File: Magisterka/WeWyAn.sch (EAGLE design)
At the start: 88 parts, among them IC1 LM324N, IC3 7805TV, IC4 LM324N, IC5 LM1117T-3.3-V, X10 22-23-2041, X11 22-23-2041, X18 22-23-2031, X19 22-23-2041, X20 22-23-2041, X21 22-23-2041, X28 22-23-2021, X29 22-23-2021, X30 22-23-2021, X31 22-23-2031, X4 22-23-2021

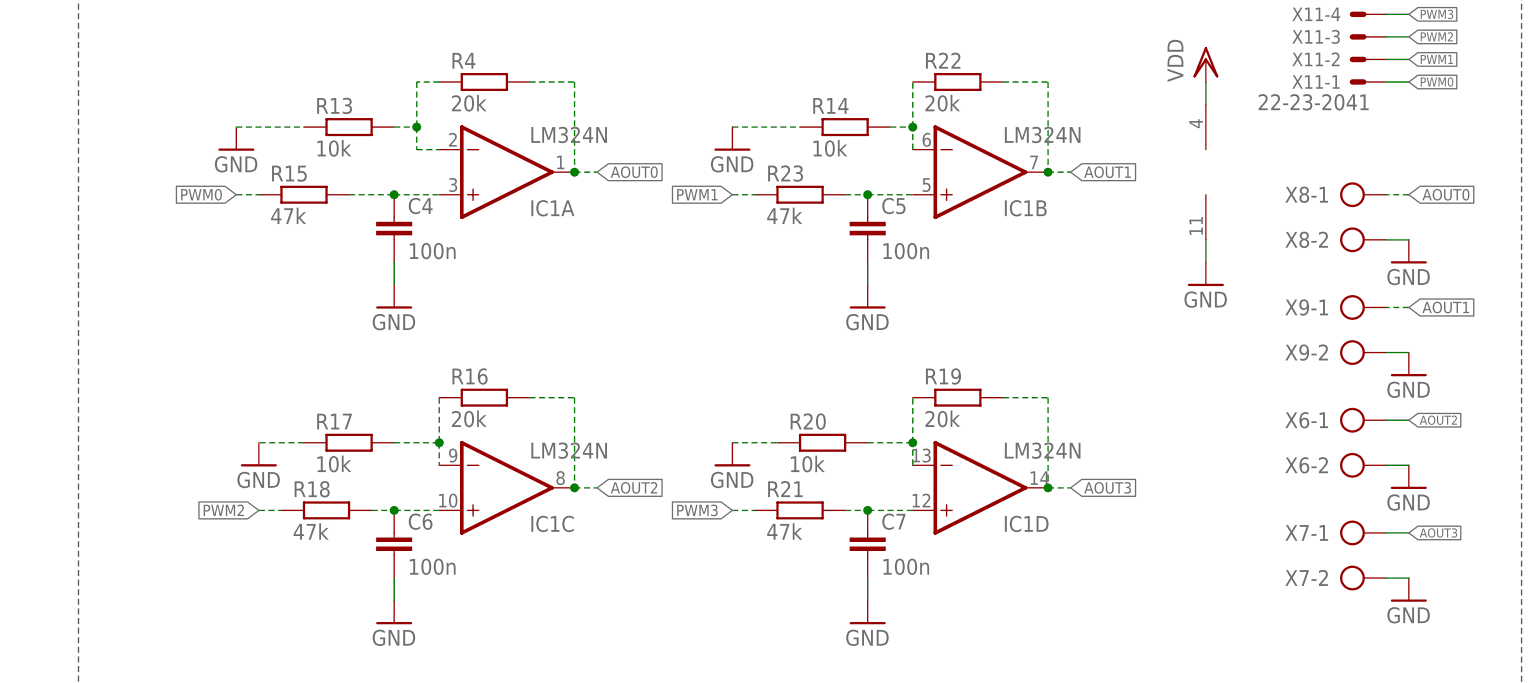
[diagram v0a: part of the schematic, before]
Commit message: size changes
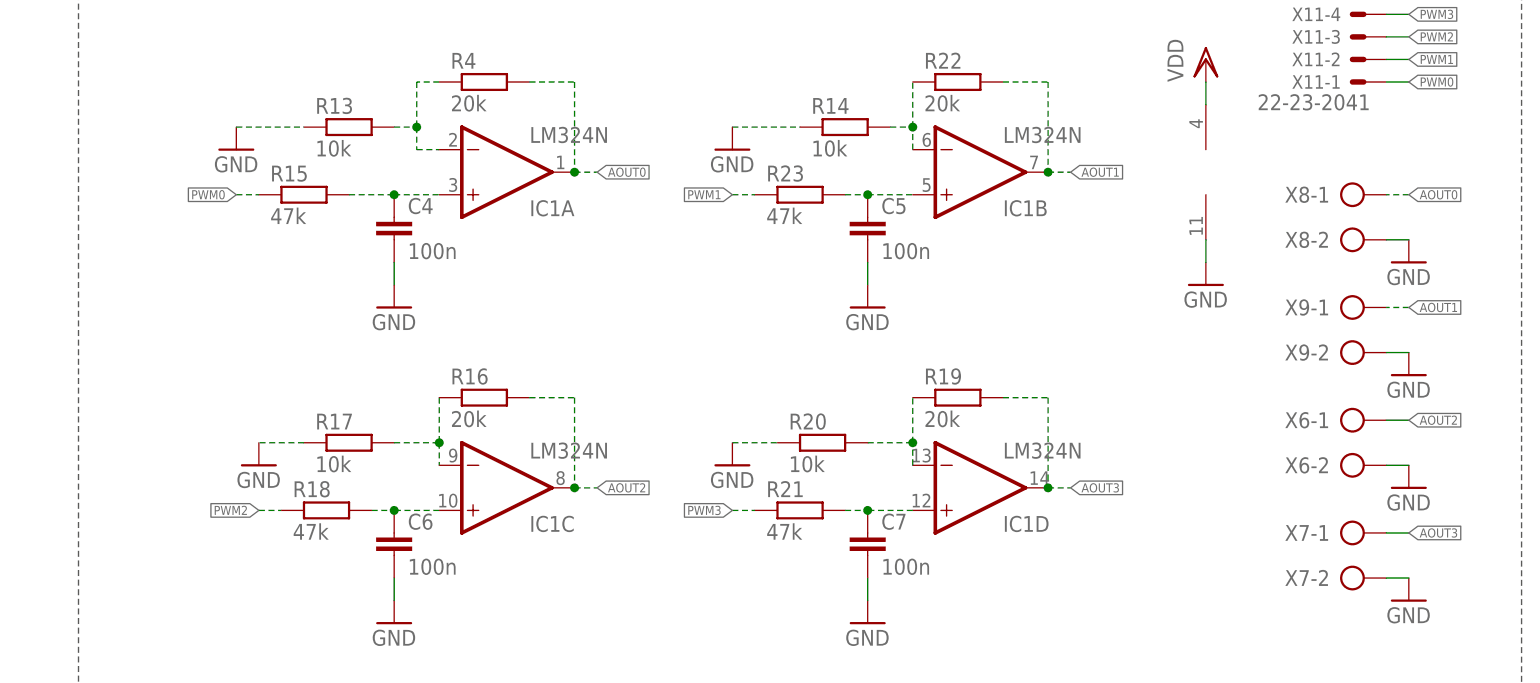
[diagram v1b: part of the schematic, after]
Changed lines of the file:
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@@
 <wire x1="261.62" y1="-30.48" x2="264.16" y2="-30.48" width="0.1524" layer="91" style="longdash"/>
 <junction x="261.62" y="-30.48"/>
-<label x="264.16" y="-30.48" size="1.27" layer="95" xref="yes"/>
+<label x="264.16" y="-30.48" size="1.016" layer="95" xref="yes"/>
 </segment>
 <segment>
 <pinref part="X8" gate="-1" pin="KL"/>
 <wire x1="355.6" y1="-33.02" x2="353.06" y2="-33.02" width="0.1524" layer="91" style="longdash"/>
-<label x="355.6" y="-33.02" size="1.27" layer="95" xref="yes"/>
+<label x="355.6" y="-33.02" size="1.016" layer="95" xref="yes"/>
 </segment>
 </net>
@@
 <pinref part="R15" gate="G$1" pin="1"/>
 <wire x1="223.52" y1="-33.02" x2="226.06" y2="-33.02" width="0.1524" layer="91" style="longdash"/>
-<label x="223.52" y="-33.02" size="1.27" layer="95" rot="R180" xref="yes"/>
+<label x="223.52" y="-33.02" size="1.016" layer="95" rot="R180" xref="yes"/>
 </segment>
 <segment>
@@
 <wire x1="261.62" y1="-66.04" x2="264.16" y2="-66.04" width="0.1524" layer="91" style="longdash"/>
 <junction x="261.62" y="-66.04"/>
-<label x="264.16" y="-66.04" size="1.27" layer="95" xref="yes"/>
+<label x="264.16" y="-66.04" size="1.016" layer="95" xref="yes"/>
 </segment>
 <segment>
@@
 <wire x1="314.96" y1="-66.04" x2="317.5" y2="-66.04" width="0.1524" layer="91" style="longdash"/>
 <junction x="314.96" y="-66.04"/>
-<label x="317.5" y="-66.04" size="1.27" layer="95" xref="yes"/>
+<label x="317.5" y="-66.04" size="1.016" layer="95" xref="yes"/>
 </segment>
 <segment>
@@
 <pinref part="R18" gate="G$1" pin="1"/>
 <wire x1="226.06" y1="-68.58" x2="228.6" y2="-68.58" width="0.1524" layer="91" style="longdash"/>
-<label x="226.06" y="-68.58" size="1.27" layer="95" rot="R180" xref="yes"/>
+<label x="226.06" y="-68.58" size="1.016" layer="95" rot="R180" xref="yes"/>
 </segment>
 <segment>
@@
 <pinref part="R21" gate="G$1" pin="1"/>
 <wire x1="279.4" y1="-68.58" x2="281.94" y2="-68.58" width="0.1524" layer="91" style="longdash"/>
-<label x="279.4" y="-68.58" size="1.27" layer="95" rot="R180" xref="yes"/>
+<label x="279.4" y="-68.58" size="1.016" layer="95" rot="R180" xref="yes"/>
 </segment>
 <segment>
@@
 <pinref part="R23" gate="G$1" pin="1"/>
 <wire x1="279.4" y1="-33.02" x2="281.94" y2="-33.02" width="0.1524" layer="91" style="longdash"/>
-<label x="279.4" y="-33.02" size="1.27" layer="95" rot="R180" xref="yes"/>
+<label x="279.4" y="-33.02" size="1.016" layer="95" rot="R180" xref="yes"/>
 </segment>
 <segment>
@@
 <wire x1="314.96" y1="-30.48" x2="317.5" y2="-30.48" width="0.1524" layer="91" style="longdash"/>
 <junction x="314.96" y="-30.48"/>
-<label x="317.5" y="-30.48" size="1.27" layer="95" xref="yes"/>
+<label x="317.5" y="-30.48" size="1.016" layer="95" xref="yes"/>
 </segment>
 <segment>
 <pinref part="X9" gate="-1" pin="KL"/>
 <wire x1="355.6" y1="-45.72" x2="353.06" y2="-45.72" width="0.1524" layer="91" style="longdash"/>
-<label x="355.6" y="-45.72" size="1.27" layer="95" xref="yes"/>
+<label x="355.6" y="-45.72" size="1.016" layer="95" xref="yes"/>
 </segment>
 </net>
